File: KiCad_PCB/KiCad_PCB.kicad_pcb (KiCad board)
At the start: 4 copper layers, 30 x 30 mm, 24 parts, among them J1 530480450, U2 NRF52832-QFAA-R, Y1 ECS-320-8-33B-7KM-TR, Y2 ECS-.327-12.5-12R-TR

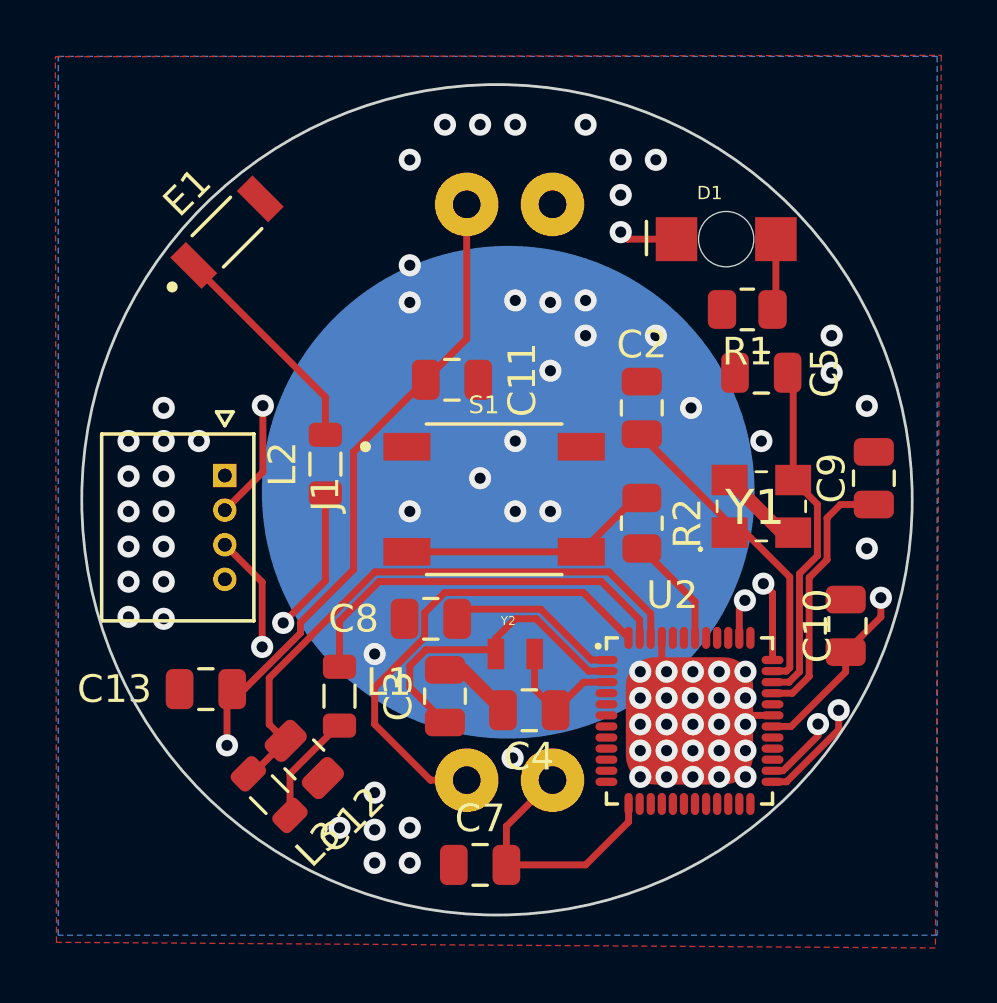
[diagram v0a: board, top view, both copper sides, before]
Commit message: Tutoría Modificacion PCB
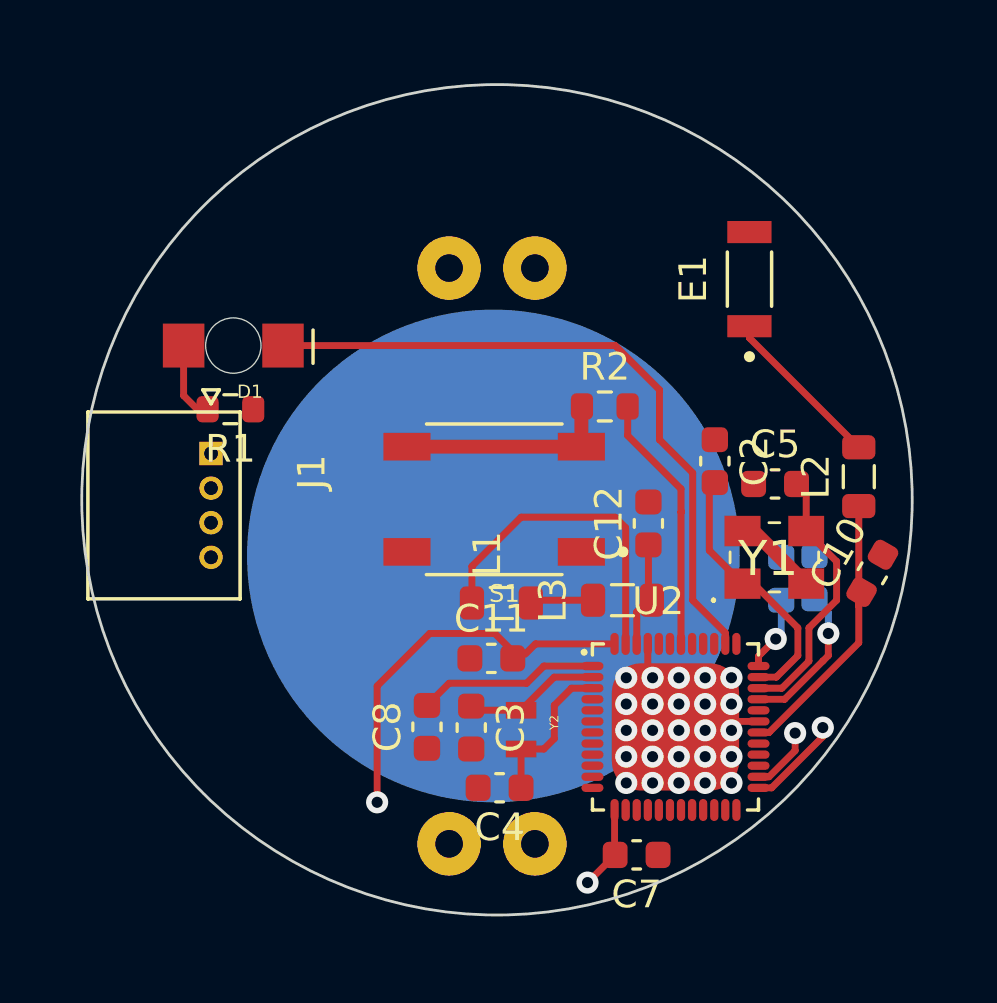
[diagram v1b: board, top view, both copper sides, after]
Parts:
- C10, C11, C12, C2, C3, C4, C5, C7, C8: footprint Capacitor_SMD:C_0805_2012Metric -> Capacitor_SMD:C_0603_1608Metric
- C13, C9: footprint Capacitor_SMD:C_0805_2012Metric -> Capacitor_SMD:C_0603_1608Metric; moved to B.Cu
- R1, R2: footprint Resistor_SMD:R_0805_2012Metric -> Resistor_SMD:R_0603_1608Metric
- moved C13 21.2 mm to (158.2, 100.2), turned to -90 degrees
- moved L2 19.3 mm to (161.0, 96.5)
- moved R1 19.0 mm to (138.3, 94.1), turned to 180 degrees
- moved E1 19.0 mm to (157.1, 89.4), turned to 90 degrees
- moved D1 18.2 mm to (138.4, 91.8), turned to 180 degrees
- moved C12 15.1 mm to (153.4, 98.2), turned to 90 degrees
- moved L3 14.6 mm to (152.5, 101.0), turned to 0 degrees
- moved C11 10.2 mm to (147.7, 103.1), turned to 0 degrees
- moved L1 6.75 mm to (148.1, 101.1), turned to 0 degrees
- moved C7 5.67 mm to (153.0, 110.2), turned to 180 degrees
- moved R2 4.43 mm to (151.8, 94.0), turned to 0 degrees
- moved C9 4.18 mm to (159.4, 100.2)
- moved C5 4.05 mm to (158.0, 96.8)
- moved C8 3.91 mm to (145.4, 105.6), turned to 90 degrees
- moved C2 3.26 mm to (155.8, 96.0)
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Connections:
- J1 pad 2: PROG_SWDIO -> PROG_SWCLK
- J1 pad 3: PROG_SWCLK -> PROG_SWDIO
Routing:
- net +1V8: track 53.4 -> 19.6 mm, vias 2 -> 3
- net Net-(C10-Pad1): track 33.9 -> 10.9 mm, vias 2 -> 0
- net Net-(C12-Pad1): track 21.2 -> 3.93 mm
- net PROG_SWDIO: track 40.5 -> 27.0 mm, vias 2 -> 1
- net Net-(C3-Pad1): track 11.6 -> 4.94 mm
- net Net-(D1-PadA): track 18.7 -> 24.4 mm, vias 2 -> 0
- net Net-(R2-Pad2): track 4.02 -> 9.41 mm
- net Net-(C9-Pad2): track 9.46 -> 5.43 mm, vias 0 -> 1
- net Net-(C5-Pad2): track 12.6 -> 9.64 mm
- net GND: track 10.2 -> 7.75 mm, vias 74 -> 25
- net Net-(L1-Pad1): track 14.3 -> 12.0 mm
- net ECS-320_XCS2: track 11.7 -> 9.59 mm
- net Net-(E1-Pad1): track 8.09 -> 6.09 mm
- net Net-(L1-Pad2): track 4.01 -> 2.12 mm
- net Net-(R2-Pad1): track 9.29 -> 7.76 mm
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- removed copper zone on In1.Cu, net +1V8
- removed copper zone on B.Cu, net GND
- removed copper zone on F.Cu, net GND
- removed copper zone on In2.Cu, net GND
